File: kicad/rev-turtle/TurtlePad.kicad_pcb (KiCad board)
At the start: 2 copper layers, 57.2 x 63.6 mm, 40 parts, among them J1 USB_IN, J2 AVR-ISP-6, SW1 SW_Push, U1 USBLC6-2SC6, U2 ATMEGA32U4, Y1 16MHz

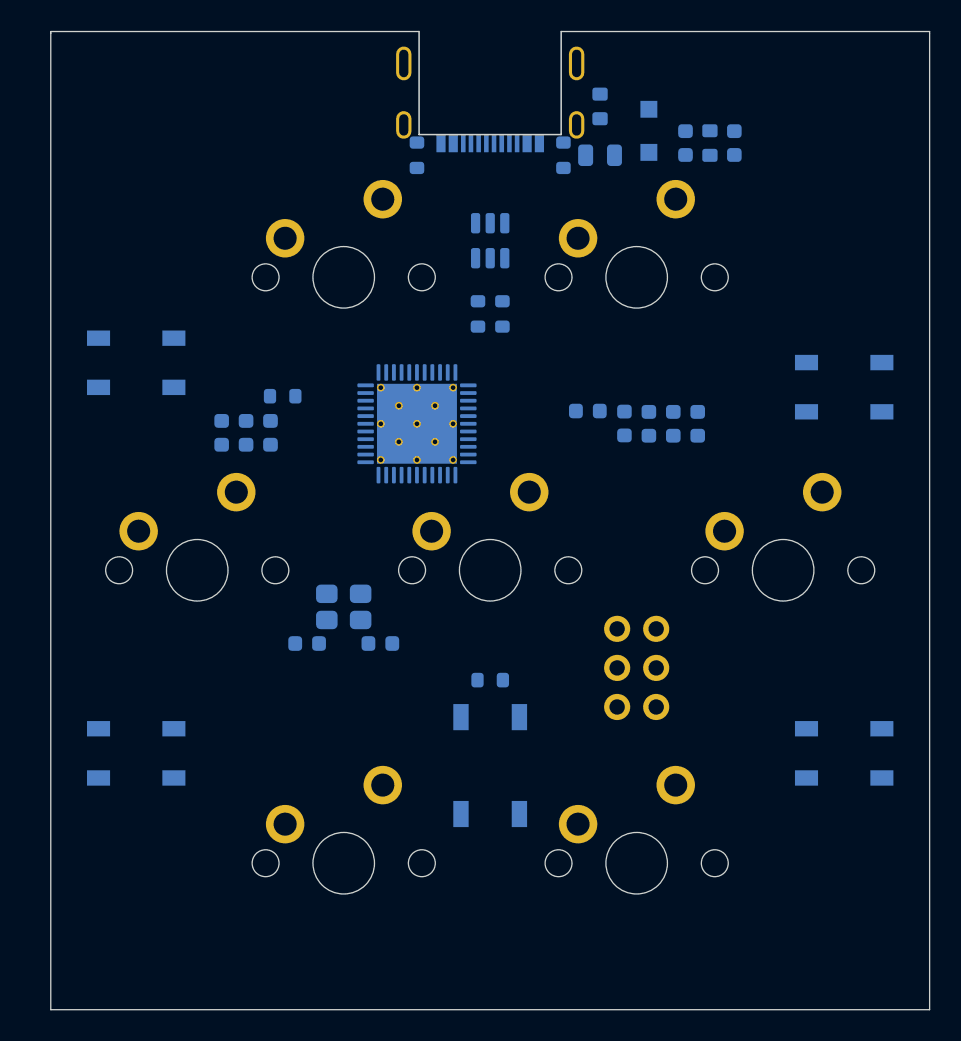
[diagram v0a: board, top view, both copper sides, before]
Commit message: Revert "Placed all surface mount parts for now"
This reverts commit df8ecd82c21d147e971f6b322fb3575a65e4f200.
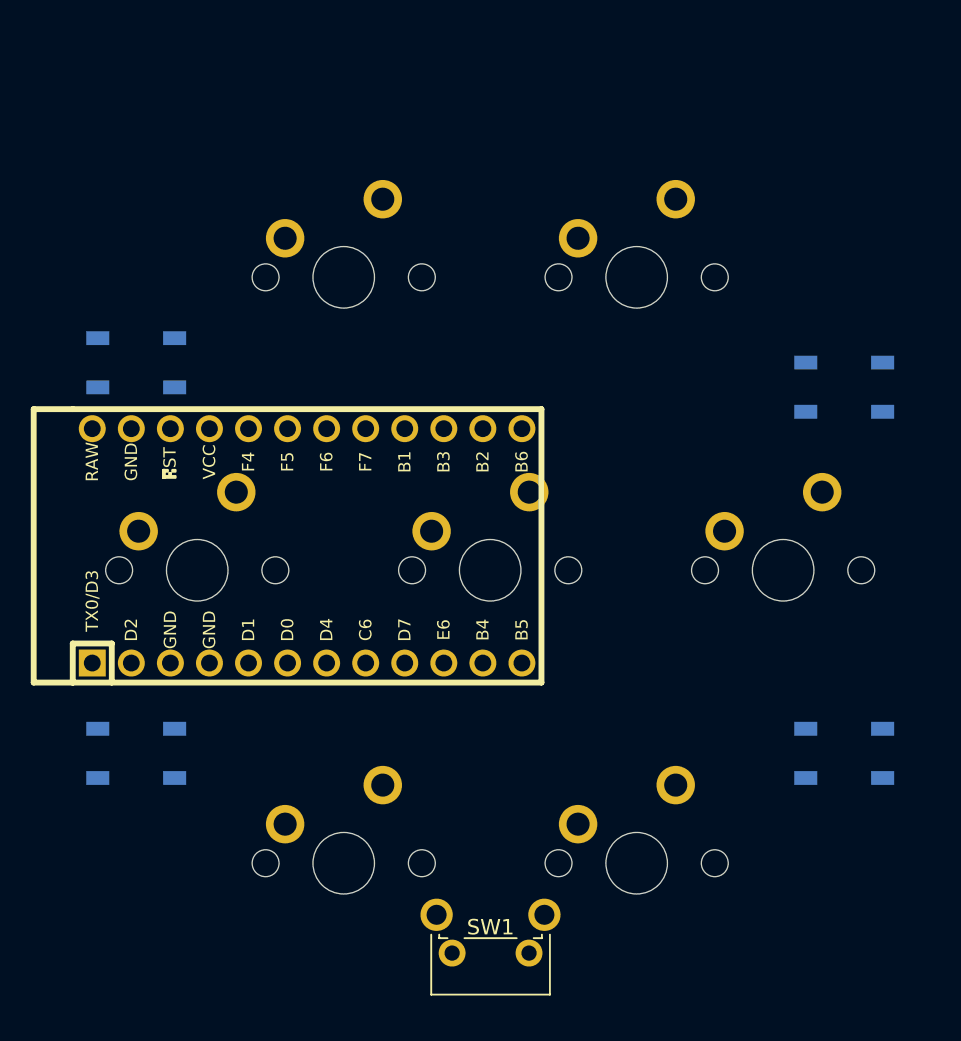
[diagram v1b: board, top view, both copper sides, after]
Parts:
- removed C1: 10u, Capacitor_SMD:C_0603_1608Metric
- removed C10, C11, C3, C4, C5, C9: 100n, Capacitor_SMD:C_0603_1608Metric
- removed C12, C2, C6: 1u, Capacitor_SMD:C_0603_1608Metric
- removed C7, C8: 22p, Capacitor_SMD:C_0603_1608Metric
- removed D1: SMF5.0CA, Diode_SMD:D_SOD-123F
- removed F1: 1A, 0xcb:Fuse_0805_2012Metric
- removed FB1, FB2: 600R, 0xcb:Ferrite_Bead_0603
- removed J1: USB_IN, 0xcb:molex2169900001
- removed J2: AVR-ISP-6, 0xcb:AVR_PROG_2.54_THT
- removed R1, R2: 5.1k, Resistor_SMD:R_0603_1608Metric
- removed R3, R4: 22, Resistor_SMD:R_0603_1608Metric
- removed R5, R6: 10k, Resistor_SMD:R_0603_1608Metric
- removed U2: ATMEGA32U4, 0xcb:QFN-44-1EP_7x7mm_P0.5mm_EP5.2x5.2mm_ThermalVias
- removed Y1: 16MHz, 0xcb:Crystal_SMD_3225-4Pin_3.2x2.5mm
- RGB1, RGB2, RGB3, RGB4: footprint LED_SMD:LED_WS2812B_PLCC4_5.0x5.0mm_P3.2mm -> Keebio-Parts:WS2812B
- SW1: footprint Button_Switch_SMD:SW_SPST_TL3342 -> Keebio-Parts:SW_Tactile_SPST_Angled_MJTP1117; moved to F.Cu
- U1: value USBLC6-2SC6 -> ProMicro; footprint Package_TO_SOT_SMD:SOT-23-6 -> Keebio-Parts:ArduinoProMicro; moved to F.Cu
- moved U1 23.1 mm to (115.9, 88.2), turned to 0 degrees
- moved SW1 12.5 mm to (130.3, 114.7), turned to 180 degrees
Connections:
- SW1 pad 1: GND -> reset
- SW1 pad 2: RST -> GND
- U1 pad 1: Net-(J1-PadA7) -> LED
- U1 pad 2: GND -> unconnected-(U1-Pad2)
- U1 pad 3: Net-(J1-PadA6) -> GND
- U1 pad 4: D+ -> GND
- U1 pad 5: /VBUS -> unconnected-(U1-Pad5)
- U1 pad 6: D- -> unconnected-(U1-Pad6)
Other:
- board outline removed

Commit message: Revert "Revert "Placed all surface mount parts for now""
This reverts commit 42bec52487df9ac41952cb28762131b75d3db880.
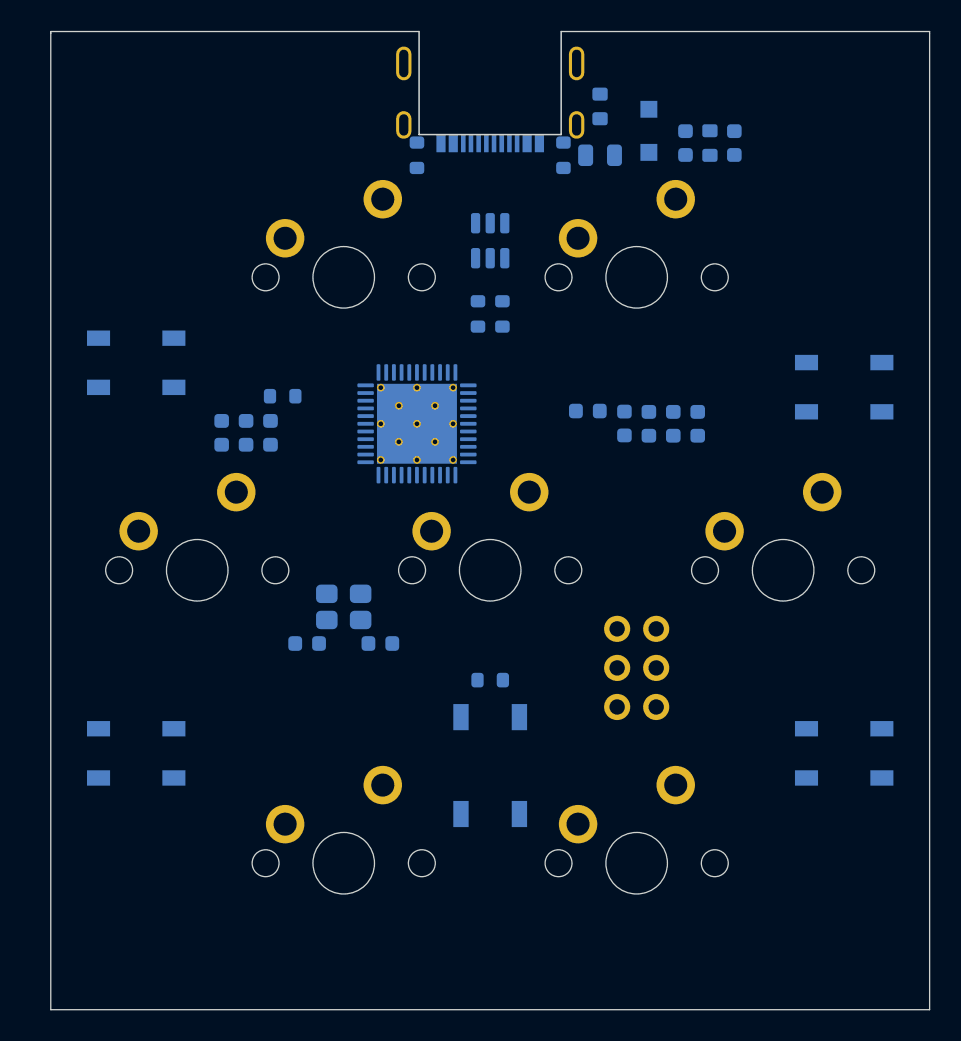
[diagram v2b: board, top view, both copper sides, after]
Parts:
- added C1: 10u, Capacitor_SMD:C_0603_1608Metric, B.Cu at (140.5, 62.0)
- added C10: 100n, Capacitor_SMD:C_0603_1608Metric, B.Cu at (110.3, 80.8)
- added C11: 100n, Capacitor_SMD:C_0603_1608Metric, B.Cu at (113.5, 80.8)
- added C12: 1u, Capacitor_SMD:C_0603_1608Metric, B.Cu at (134.1, 79.4)
- added C2: 1u, Capacitor_SMD:C_0603_1608Metric, B.Cu at (143.7, 62.0)
- added C3: 100n, Capacitor_SMD:C_0603_1608Metric, B.Cu at (139.7, 80.3)
- added C4: 100n, Capacitor_SMD:C_0603_1608Metric, B.Cu at (138.1, 80.3)
- added C5: 100n, Capacitor_SMD:C_0603_1608Metric, B.Cu at (136.5, 80.2)
- added C6: 1u, Capacitor_SMD:C_0603_1608Metric, B.Cu at (141.3, 80.3)
- added C7: 22p, Capacitor_SMD:C_0603_1608Metric, B.Cu at (120.7, 94.5)
- added C8: 22p, Capacitor_SMD:C_0603_1608Metric, B.Cu at (115.9, 94.5)
- added C9: 100n, Capacitor_SMD:C_0603_1608Metric, B.Cu at (111.9, 80.8)
- added D1: SMF5.0CA, Diode_SMD:D_SOD-123F, B.Cu at (138.1, 61.2)
- added F1: 1A, 0xcb:Fuse_0805_2012Metric, B.Cu at (134.9, 62.8)
- added FB1: 600R, 0xcb:Ferrite_Bead_0603, B.Cu at (142.1, 62.0)
- added FB2: 600R, 0xcb:Ferrite_Bead_0603, B.Cu at (134.9, 59.6)
- added J1: USB_IN, 0xcb:molex2169900001, B.Cu at (127.8, 54.7)
- added J2: AVR-ISP-6, 0xcb:AVR_PROG_2.54_THT, B.Cu at (137.3, 96.1)
- added R1: 5.1k, Resistor_SMD:R_0603_1608Metric, B.Cu at (123.0, 62.8)
- added R2: 5.1k, Resistor_SMD:R_0603_1608Metric, B.Cu at (132.6, 62.8)
- added R3: 22, Resistor_SMD:R_0603_1608Metric, B.Cu at (128.6, 73.1)
- added R4: 22, Resistor_SMD:R_0603_1608Metric, B.Cu at (127.0, 73.1)
- added R5: 10k, Resistor_SMD:R_0603_1608Metric, B.Cu at (127.8, 96.9)
- added R6: 10k, Resistor_SMD:R_0603_1608Metric, B.Cu at (114.3, 78.5)
- added U2: ATMEGA32U4, 0xcb:QFN-44-1EP_7x7mm_P0.5mm_EP5.2x5.2mm_ThermalVias, B.Cu at (123.0, 80.3)
- added Y1: 16MHz, 0xcb:Crystal_SMD_3225-4Pin_3.2x2.5mm, B.Cu at (118.3, 92.2)
- RGB1, RGB2, RGB3, RGB4: footprint Keebio-Parts:WS2812B -> LED_SMD:LED_WS2812B_PLCC4_5.0x5.0mm_P3.2mm
- SW1: footprint Keebio-Parts:SW_Tactile_SPST_Angled_MJTP1117 -> Button_Switch_SMD:SW_SPST_TL3342; moved to B.Cu
- U1: value ProMicro -> USBLC6-2SC6; footprint Keebio-Parts:ArduinoProMicro -> Package_TO_SOT_SMD:SOT-23-6; moved to B.Cu
- moved U1 23.1 mm to (127.8, 68.3), turned to -90 degrees
- moved SW1 12.5 mm to (127.8, 102.5), turned to -90 degrees
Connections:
- SW1 pad 1: reset -> GND
- SW1 pad 2: GND -> RST
- U1 pad 1: LED -> Net-(J1-PadA7)
- U1 pad 2: unconnected-(U1-Pad2) -> GND
- U1 pad 3: GND -> Net-(J1-PadA6)
- U1 pad 4: GND -> D+
- U1 pad 5: unconnected-(U1-Pad5) -> /VBUS
- U1 pad 6: unconnected-(U1-Pad6) -> D-
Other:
- board outline added: 57.2 x 63.6 mm
